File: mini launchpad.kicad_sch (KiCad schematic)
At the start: 144 parts, among them J1 Conn_01x08_Socket, J2 Conn_01x06_Socket, J3 Conn_01x02_Pin, J4 AudioJack3_Ground, P1 USB_C_Plug_USB2.0, Q1 AO3401A, SW65 SW_DPDT_x2, SW66 RotaryEncoder_Switch_MP, SW67 RotaryEncoder_Switch_MP, SW68 RotaryEncoder_Switch_MP, SW69 RotaryEncoder_Switch_MP, SW70 RotaryEncoder_Switch_MP, SW71 RotaryEncoder_Switch_MP, SW72 RotaryEncoder_Switch_MP, SW73 RotaryEncoder_Switch_MP, SW75 SW_Push, SW76 SW_Push, SW77 SW_Push, SW78 SW_Push, SW79 SW_Push, SW80 SW_Push, SW81 SW_Push, SW83 SW_Push, U1 MCP23017_ML, U10 W25Q128JVS, U11 MCP23017_ML, U12 LM386, U13 LM386, U2 MCP23017_ML, U3 MCP23017_ML, U4 MCP23017_ML, U5 CP2615-xx-xM, U6 TMUX1574PW, U7 CH334R, U8 RP2040, U9 NCP1117-3.3_TO252, Y1 12MHz

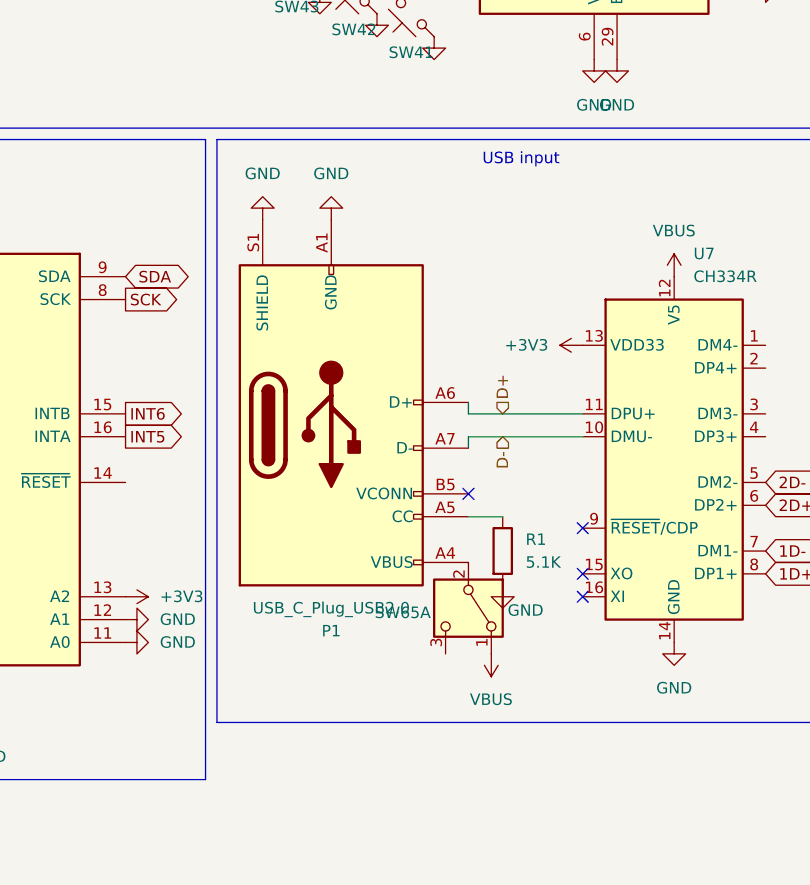
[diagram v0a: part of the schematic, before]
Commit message: pcb update
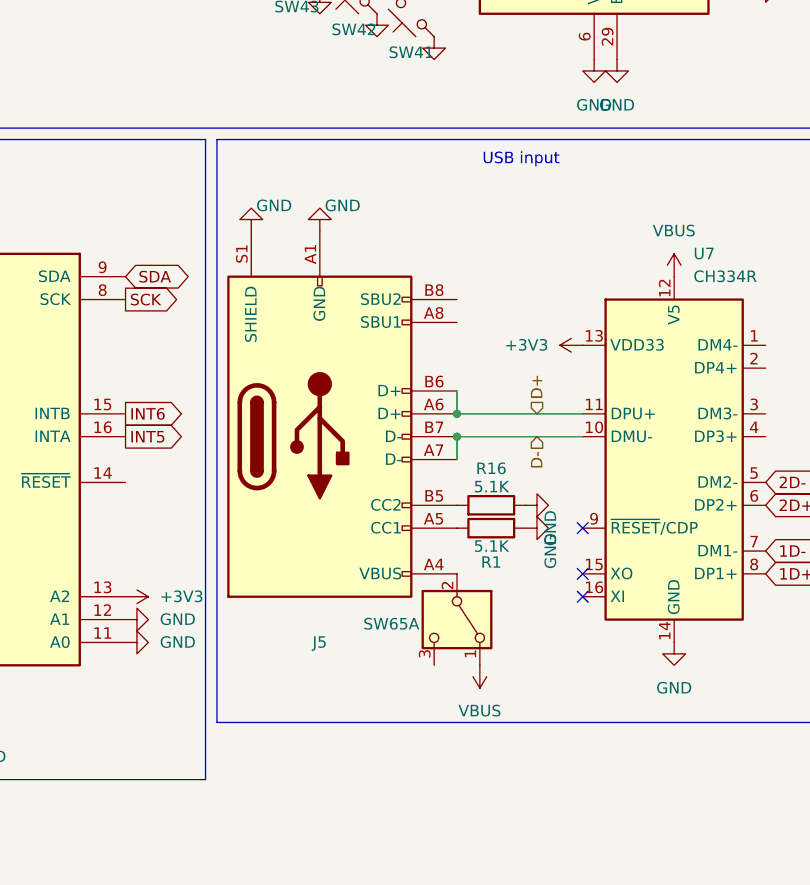
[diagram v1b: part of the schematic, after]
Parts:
- removed P1: USB_C_Plug_USB2.0, Connector_USB:USB_C_Plug_JAE_DX07P024AJ1, symbol Connector:USB_C_Plug_USB2.0
- added J5: USB_C_Receptacle_USB2.0_16P, Connector_USB:USB_C_Receptacle_Amphenol_124019772112A, symbol Connector:USB_C_Receptacle_USB2.0_16P
- added R16: 5.1K, Resistor_SMD:R_0402_1005Metric, symbol Device:R
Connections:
- net D+: now also J5.A6 (D+), J5.B6 (D+)
- net D-: now also J5.A7 (D-), J5.B7 (D-)
- net GND: now also J5.A1 (GND), J5.A12 (GND), J5.B1 (GND), J5.B12 (GND), J5.S1 (SHIELD), R16.1
- net at R1.1: now also J5.A5 (CC1)
- net at SW65.2 (B): now also J5.A4 (VBUS), J5.A9 (VBUS), J5.B4 (VBUS), J5.B9 (VBUS)
- new net: J5.B5 (CC2), R16.2
- no-connect marks 7 -> 6
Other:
- moved on the sheet: R1, SW65A
